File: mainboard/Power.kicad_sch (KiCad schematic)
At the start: 32 parts, among them IC801 TPS62823DLC, IC802 LP5907MFX-2.8, IC803 LP5907MFX-1.5, IC804 LP5907MFX-3.0, IC805 LP5907MFX-2.8, IC806 LP5907MFX-1.2

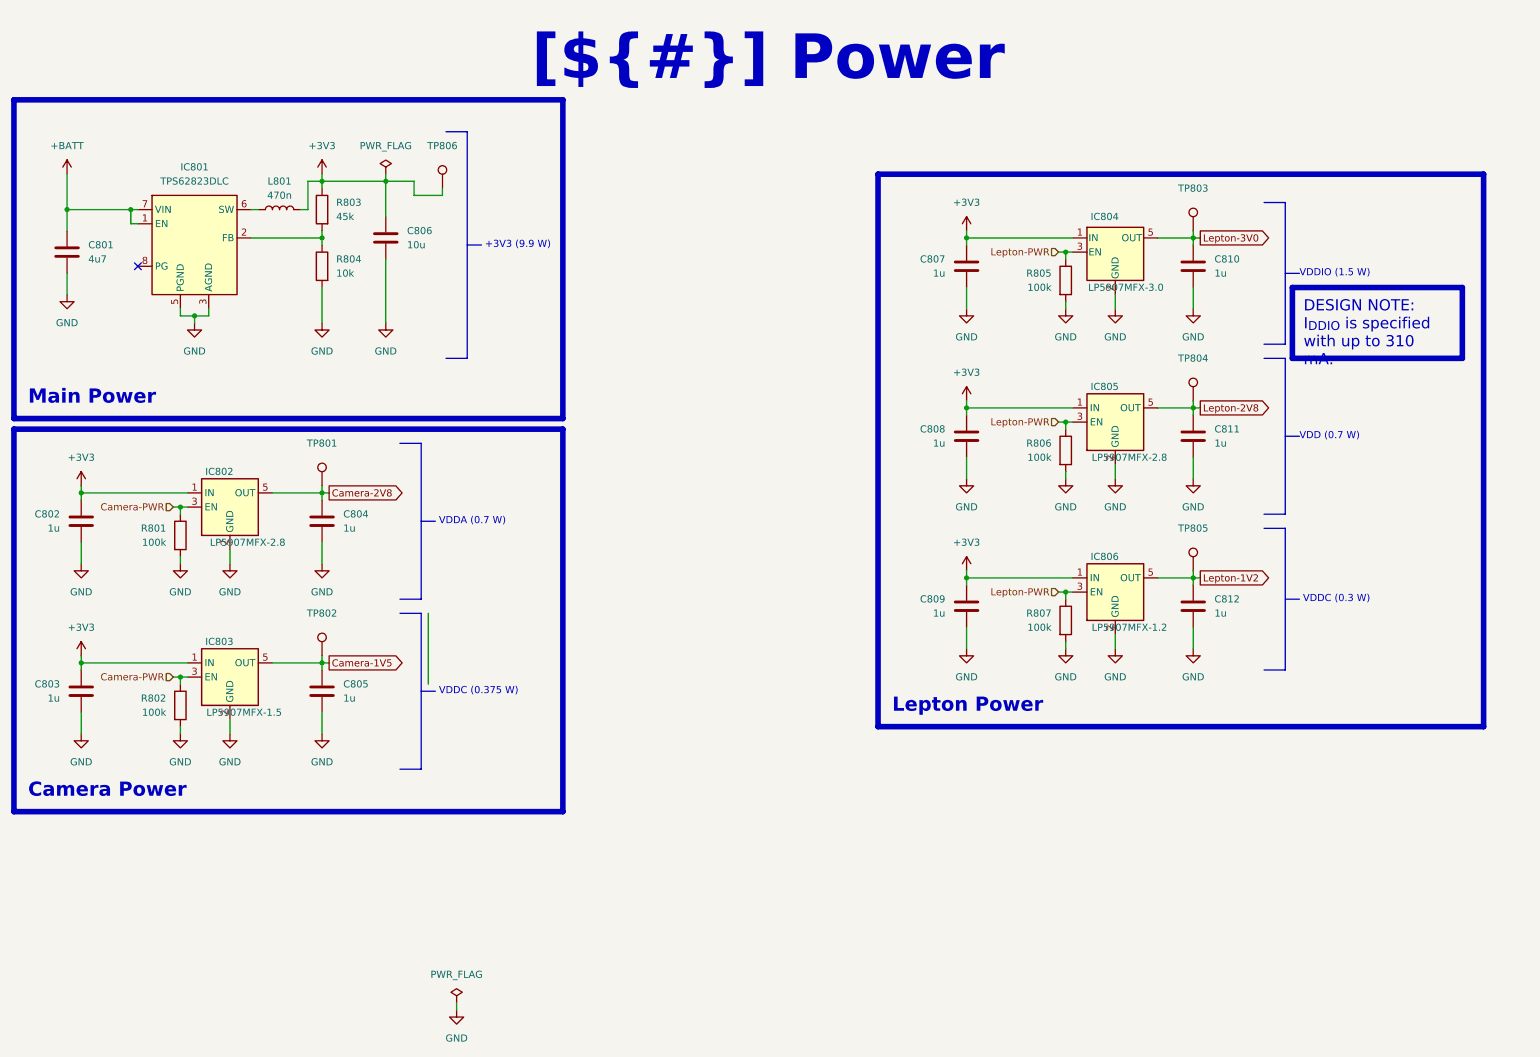
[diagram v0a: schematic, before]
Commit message: Layout complete
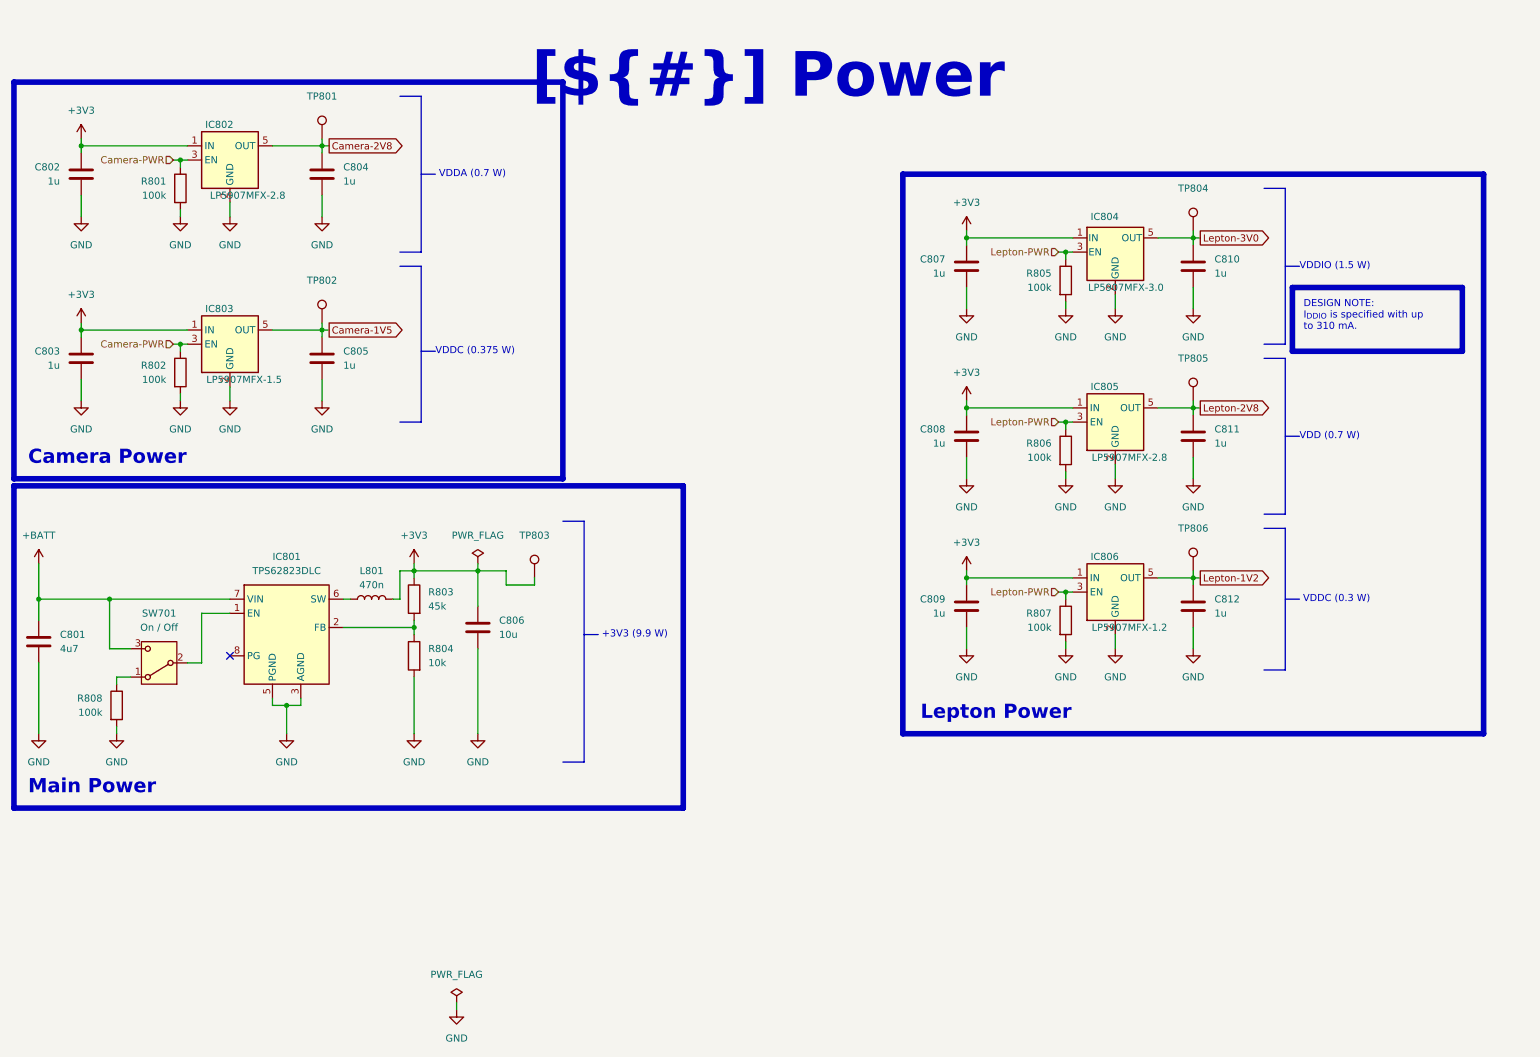
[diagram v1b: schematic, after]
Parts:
- added R808: 100k, Resistor_SMD:R_0603_1608Metric, symbol Device:R
- added SW701: On / Off, Button_Switch_THT:SW_Slide_SPDT_Angled_CK_OS102011MA1Q, symbol Switch:SW_SPDT
- renumbered TP806 to TP803, TP803 to TP804, TP804 to TP805, TP805 to TP806
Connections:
- net +BATT: now also SW701.3 (C); no longer IC801.1 (EN)
- net GND: now also R808.2
- new net: IC801.1 (EN), SW701.2 (B)
- new net: R808.1, SW701.1 (A)
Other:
- moved on the sheet: C801, C802, C803, C804, C805, C806, IC801, IC802, IC803, L801, R801, R802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

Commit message: Release 1.0.0
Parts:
- TP801, TP802, TP803, TP804, TP805, TP806: footprint TestPoint:TestPoint_Pad_1.0x1.0mm -> Testpoints_Kampi:TestPoint_Pad_1.0x1.0mm
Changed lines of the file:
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@@
 			)
 		)
-		(property "Footprint" "TestPoint:TestPoint_Pad_1.0x1.0mm"
+		(property "Footprint" "Testpoints_Kampi:TestPoint_Pad_1.0x1.0mm"
 			(at 111.76 113.03 0)
 			(effects
@@
 			)
 		)
-		(property "Footprint" "TestPoint:TestPoint_Pad_1.0x1.0mm"
+		(property "Footprint" "Testpoints_Kampi:TestPoint_Pad_1.0x1.0mm"
 			(at 229.87 81.28 0)
 			(effects
@@
 			)
 		)
-		(property "Footprint" "TestPoint:TestPoint_Pad_1.0x1.0mm"
+		(property "Footprint" "Testpoints_Kampi:TestPoint_Pad_1.0x1.0mm"
 			(at 73.66 34.29 0)
 			(effects
@@
 			)
 		)
-		(property "Footprint" "TestPoint:TestPoint_Pad_1.0x1.0mm"
+		(property "Footprint" "Testpoints_Kampi:TestPoint_Pad_1.0x1.0mm"
 			(at 229.87 111.76 0)
 			(effects
@@
 			)
 		)
-		(property "Footprint" "TestPoint:TestPoint_Pad_1.0x1.0mm"
+		(property "Footprint" "Testpoints_Kampi:TestPoint_Pad_1.0x1.0mm"
 			(at 229.87 50.8 0)
 			(effects
@@
 			)
 		)
-		(property "Footprint" "TestPoint:TestPoint_Pad_1.0x1.0mm"
+		(property "Footprint" "Testpoints_Kampi:TestPoint_Pad_1.0x1.0mm"
 			(at 73.66 67.31 0)
 			(effects
